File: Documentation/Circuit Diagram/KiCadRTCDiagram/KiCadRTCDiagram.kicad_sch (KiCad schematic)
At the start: 4 parts, among them IC1 DS3231

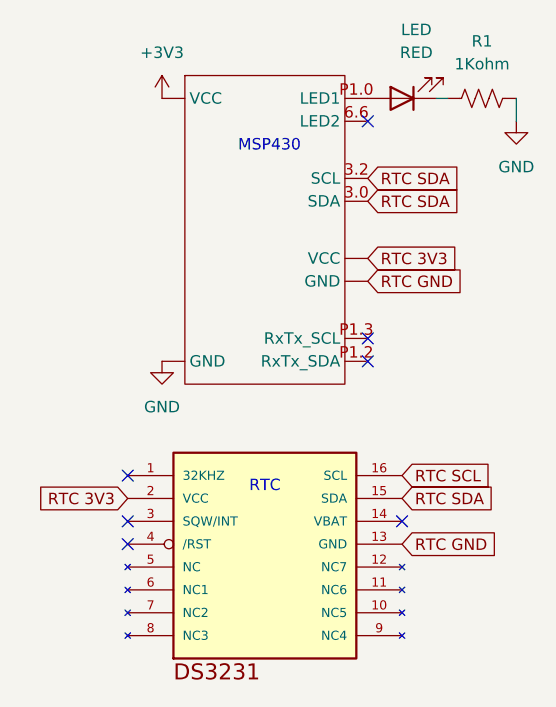
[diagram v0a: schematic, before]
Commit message: completed documentation
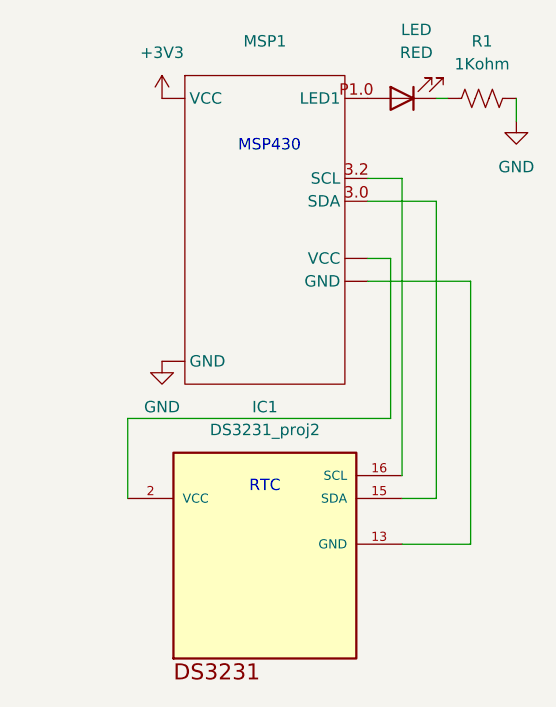
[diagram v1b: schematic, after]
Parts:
- removed IC1: DS3231, DS3231:SO16W, symbol RTC:DS3231
- removed MSP1: ~, symbol msp430fr2355:MSP430FR2355
- added IC1: DS3231_proj2, DS3231:SO16W, symbol RTC:DS3231_proj2
- added MSP1: ~, symbol RTC:MSP430FR2355_proj2
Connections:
- net +3V3: now also MSP1. (VCC)
- net GND: now also MSP1. (VCC)
- net at LED.2 (A): now also MSP1.P1.0 (LED1)
- new net: IC1.13 (GND), MSP1. (VCC)
- new net: IC1.15 (SDA), MSP1.3.0 (SDA)
- new net: IC1.16 (SCL), MSP1.3.2 (SCL)
- new net: IC1.2 (VCC), MSP1. (VCC)
- no-connect marks 7 -> 0
